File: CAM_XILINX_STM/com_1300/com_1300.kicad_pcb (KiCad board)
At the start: 4 copper layers, 50 x 75.9 mm, 95 parts, among them IC1 XC3S400-4TQ144C, J1 Conn_02x04_Top_Bottom, J2 Conn_02x04_Top_Bottom, J3 9-68RD-0.635SF, U1 LT1963AxST-3.3, U2 LP3982IMM-ADJ, U3 LTC3411EMS, U4 STM32F415RGTx, U5 AM29LV320DT90EC, U6 TC74LCX373FT, Y1 40mHZ, Y2 16mHz

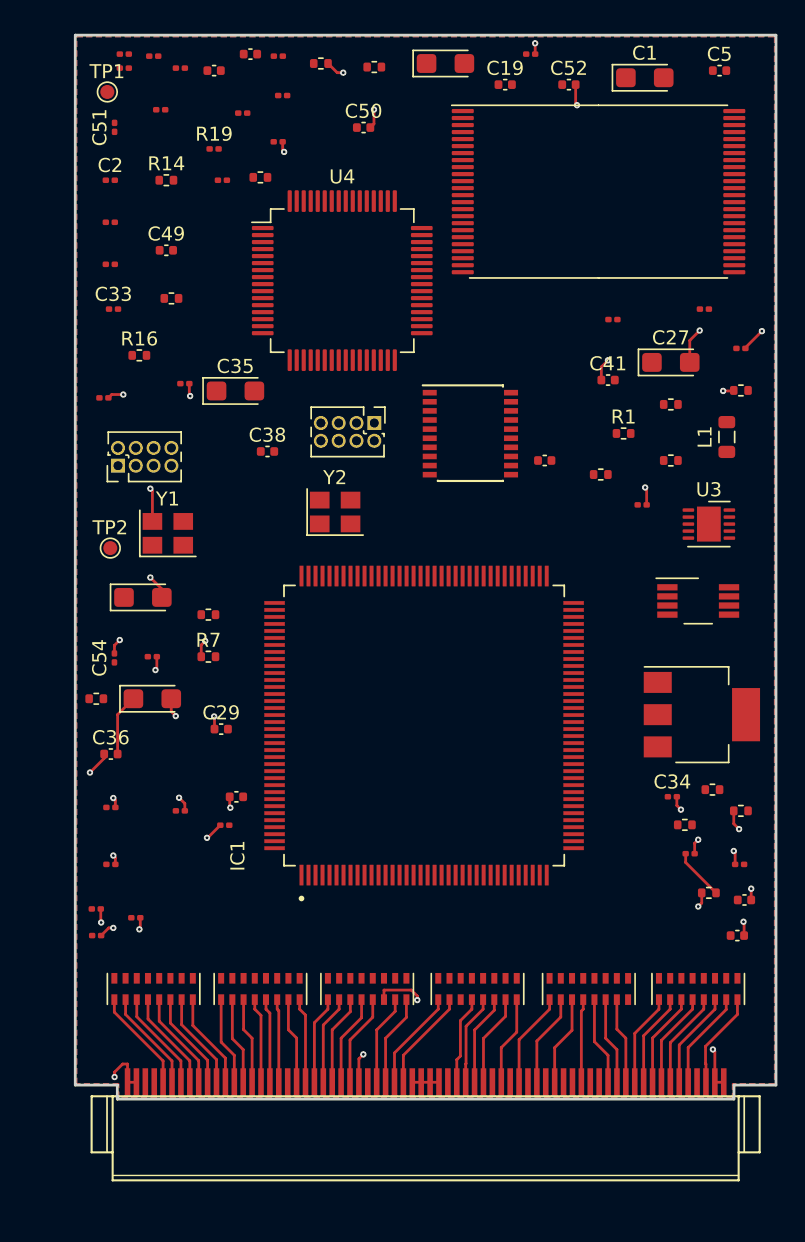
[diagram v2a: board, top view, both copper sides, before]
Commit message: tracert
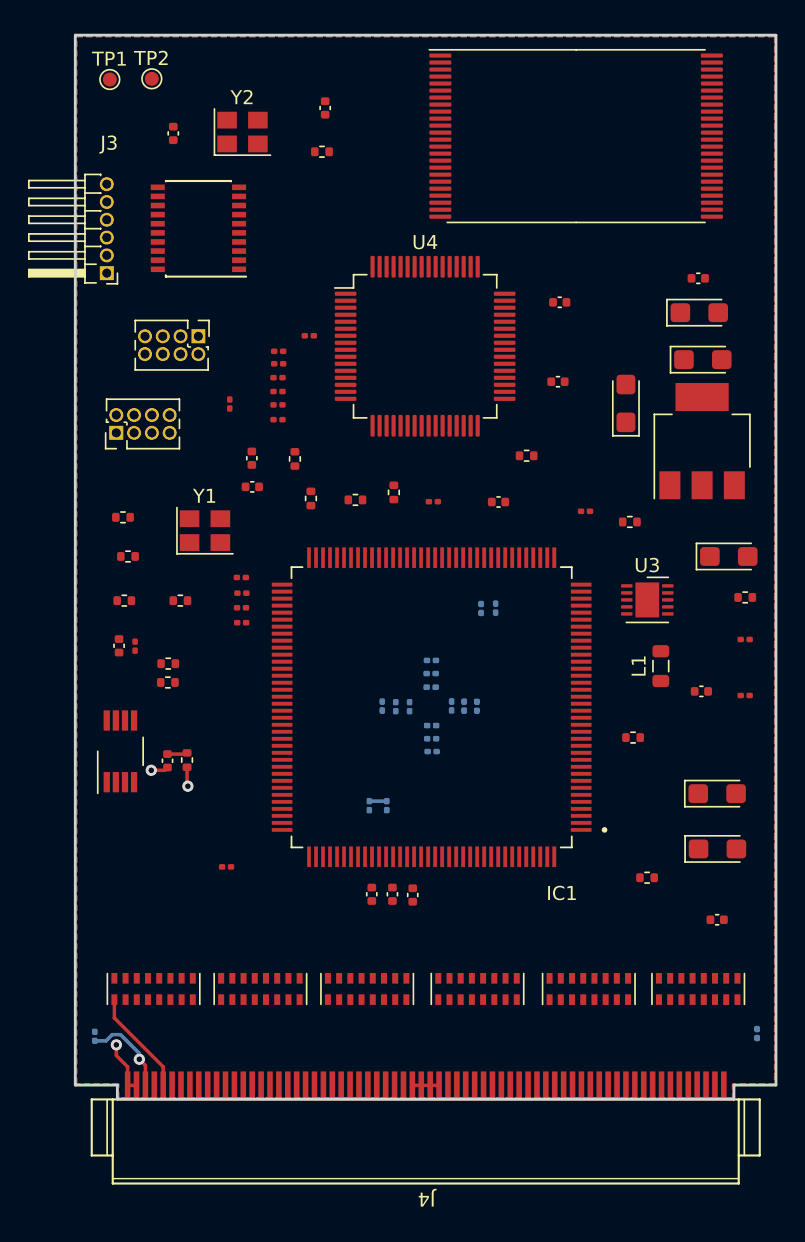
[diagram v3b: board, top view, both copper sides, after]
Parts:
- added J4: 9-68RD-0.635SF, PC_Card:IC9_Series, F.Cu at (57.5, 99.6)
- C24 (x16), R19: moved to B.Cu
- J3: value 9-68RD-0.635SF -> Conn_02x03_Top_Bottom; footprint PC_Card:IC9_Series -> Connector_PinHeader_1.27mm:PinHeader_1x06_P1.27mm_Horizontal
- R18: footprint Resistor_SMD:R_0402_1005Metric -> Resistor_SMD:R_0201_0603Metric; moved to B.Cu
- moved R18 75.9 mm to (81.2, 94.9), turned to 90 degrees
- moved R19 63.9 mm to (33.9, 95.1), turned to -90 degrees
- moved J3 63.0 mm to (34.7, 40.6)
- moved C26 60.9 mm to (80.3, 66.8)
- moved C5 59.3 mm to (35.6, 67.2), turned to -90 degrees
- moved C24 52.6 mm to (57.9, 73.9), turned to 180 degrees
- moved C24 49.5 mm to (59.4, 71.5), turned to 90 degrees
- moved C24 49.2 mm to (57.9, 70.2), turned to 180 degrees
- moved C4 49.0 mm to (43.3, 83.0)
- moved C36 44.8 mm to (78.3, 86.8)
- moved C35 44.8 mm to (78.3, 77.8)
- moved C24 44.8 mm to (57.9, 69.2), turned to 180 degrees
- moved C25 44.6 mm to (77.0, 43.5)
- moved C24 44.4 mm to (55.4, 71.6), turned to 90 degrees
- moved C24 43.8 mm to (57.9, 68.3), turned to 180 degrees
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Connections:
- net uC_PROG4 renamed uC_MOSI
- IC1 pad 10: INOUT_A4 -> INOUT_MDI4
- IC1 pad 100: INOUT_MDI4 -> INOUT_A4
- IC1 pad 102: INOUT_MDI5 -> INOUT_A5
- IC1 pad 103: INOUT_MDI6 -> INOUT_A6
- IC1 pad 104: INOUT_MDI7 -> INOUT_A7
- IC1 pad 105: INOUT_MCLKI -> INOUT_MCLKO
- IC1 pad 11: INOUT_A3 -> INOUT_MDI3
- IC1 pad 12: INOUT_A2 -> INOUT_MDI2
- IC1 pad 13: INOUT_A1 -> INOUT_MDI1
- IC1 pad 14: INOUT_A0 -> INOUT_MDI0
- IC1 pad 15: INOUT_INPACK# -> INOUT_CE1#
- IC1 pad 17: INOUT_REG# -> INOUT_OE#
- IC1 pad 21: INOUT_MOVAL -> INOUT_MOSTRT
- IC1 pad 23: INOUT_MIVAL -> INOUT_D7
- IC1 pad 24: INOUT_MDO7 -> INOUT_D6
- IC1 pad 25: INOUT_MDO6 -> INOUT_D5
- IC1 pad 26: INOUT_MDO5 -> INOUT_D4
- IC1 pad 27: INOUT_MDO4 -> INOUT_D3
- IC1 pad 28: INOUT_MDO3 -> INOUT_D2
- IC1 pad 30: INOUT_MDO2 -> INOUT_D1
- IC1 pad 31: INOUT_MDO1 -> INOUT_D0
- IC1 pad 32: INOUT_MDO0 -> INOUT_IREQ#
- IC1 pad 33: INOUT_IREQ# -> unconnected-(IC1-IO_L20N_6-Pad33)
- IC1 pad 5: INOUT_MCLKO -> INOUT_MCLKI
- IC1 pad 6: INOUT_A7 -> INOUT_MDI7
- IC1 pad 7: INOUT_A6 -> INOUT_MDI6
- IC1 pad 76: unconnected-(IC1-IO_1-Pad76) -> INOUT_MDO0
- IC1 pad 77: INOUT_D0 -> INOUT_MDO1
- IC1 pad 78: INOUT_D1 -> INOUT_MDO2
- IC1 pad 79: INOUT_D2 -> INOUT_MDO3
- IC1 pad 8: INOUT_A5 -> INOUT_MDI5
- IC1 pad 80: INOUT_D3 -> INOUT_MDO4
- IC1 pad 82: INOUT_D4 -> INOUT_MDO5
- IC1 pad 83: INOUT_D5 -> INOUT_MDO6
- IC1 pad 85: INOUT_D6 -> INOUT_MDO7
- IC1 pad 86: INOUT_D7 -> INOUT_MIVAL
- IC1 pad 87: INOUT_MOSTRT -> INOUT_MOVAL
- IC1 pad 89: INOUT_OE# -> INOUT_REG#
- IC1 pad 93: INOUT_CE1# -> INOUT_INPACK#
- IC1 pad 95: INOUT_MDI0 -> INOUT_A0
- IC1 pad 96: INOUT_MDI1 -> INOUT_A1
- IC1 pad 97: INOUT_MDI2 -> INOUT_A2
- IC1 pad 99: INOUT_MDI3 -> INOUT_A3
- J2 pad 3: uC_PROG1 -> uC_MISO
- J2 pad 4: uC_PROG2 -> uC_SCK
- J3 pad 1: GND -> +3V3
- J3 pad 2: D3 -> BOOT0
- J3 pad 3: D4 -> SWIDO
- J3 pad 4: D5 -> GND
- J3 pad 5: D6 -> unconnected-(J3-Pin_5-Pad5)
- J3 pad 6: D7 -> SWCLK
- R18 pad 1: Net-(J3-CD1#) -> Net-(J4-CD1#)
- R19 pad 2: Net-(J3-CD2#) -> Net-(J4-CD2#)
- U4 pad 10: uC_PROG1 -> uC_MISO
- U4 pad 29: uC_PROG2 -> uC_SCK
- U4 pad 46: unconnected-(U4-PA13-Pad46) -> SWIDO
- U4 pad 49: unconnected-(U4-PA14-Pad49) -> SWCLK
- U4 pad 60: unconnected-(U4-BOOT0-Pad60) -> BOOT0
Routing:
- net GND: track 48.9 -> 6.48 mm, vias 37 -> 3
- net MDI6: track 11.1 -> 0.00 mm, vias 2 -> 0
- net D2: track 7.27 -> 0.00 mm
- net MIVAL: track 7.26 -> 0.00 mm
- net MDO1: track 7.20 -> 0.00 mm
- net MDI4: track 7.19 -> 0.00 mm
- net D1: track 7.13 -> 0.00 mm
- net MDO0: track 7.07 -> 0.00 mm
- net D4: track 7.02 -> 0.00 mm
- net D0: track 7.00 -> 0.00 mm
- net MDO3: track 6.96 -> 0.00 mm
- net MOSTRT: track 6.93 -> 0.00 mm
- net D5: track 6.89 -> 0.00 mm
- net A0: track 6.86 -> 0.00 mm
- net D3: track 6.85 -> 0.00 mm
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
